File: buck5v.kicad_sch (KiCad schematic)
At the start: 11 parts, among them U4 LM76005

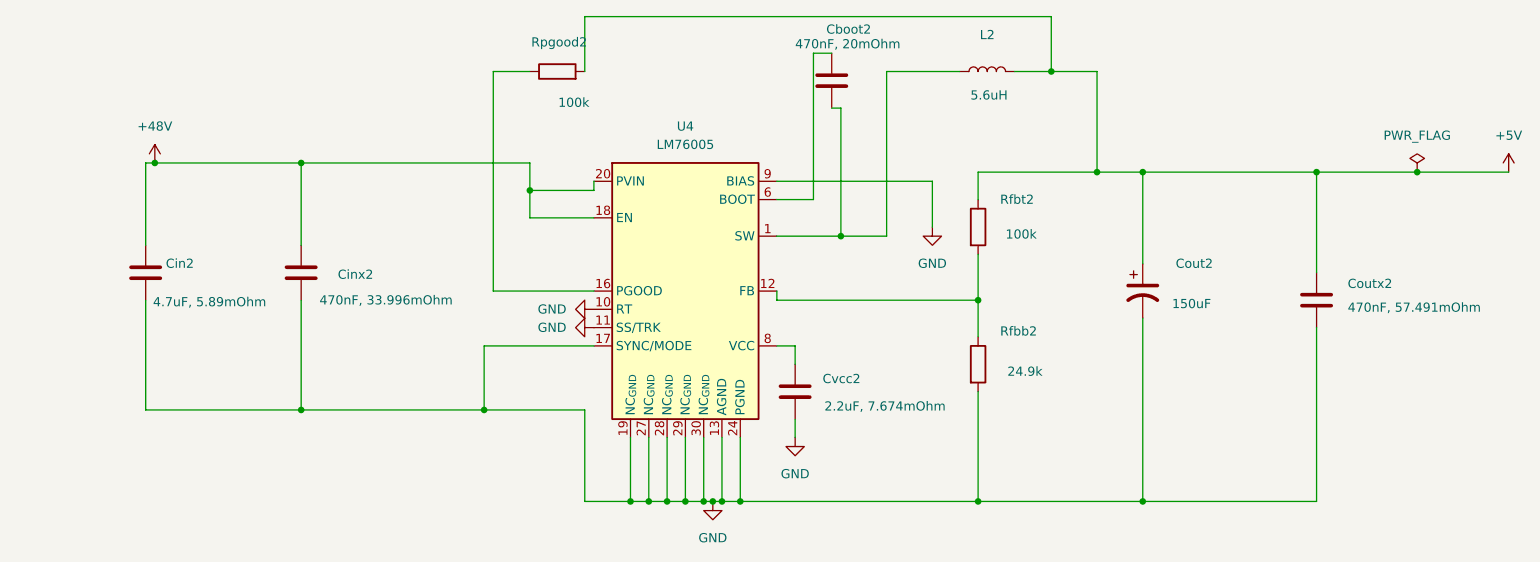
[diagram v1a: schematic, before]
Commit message: Fixed Schematics with more cost effective IC's
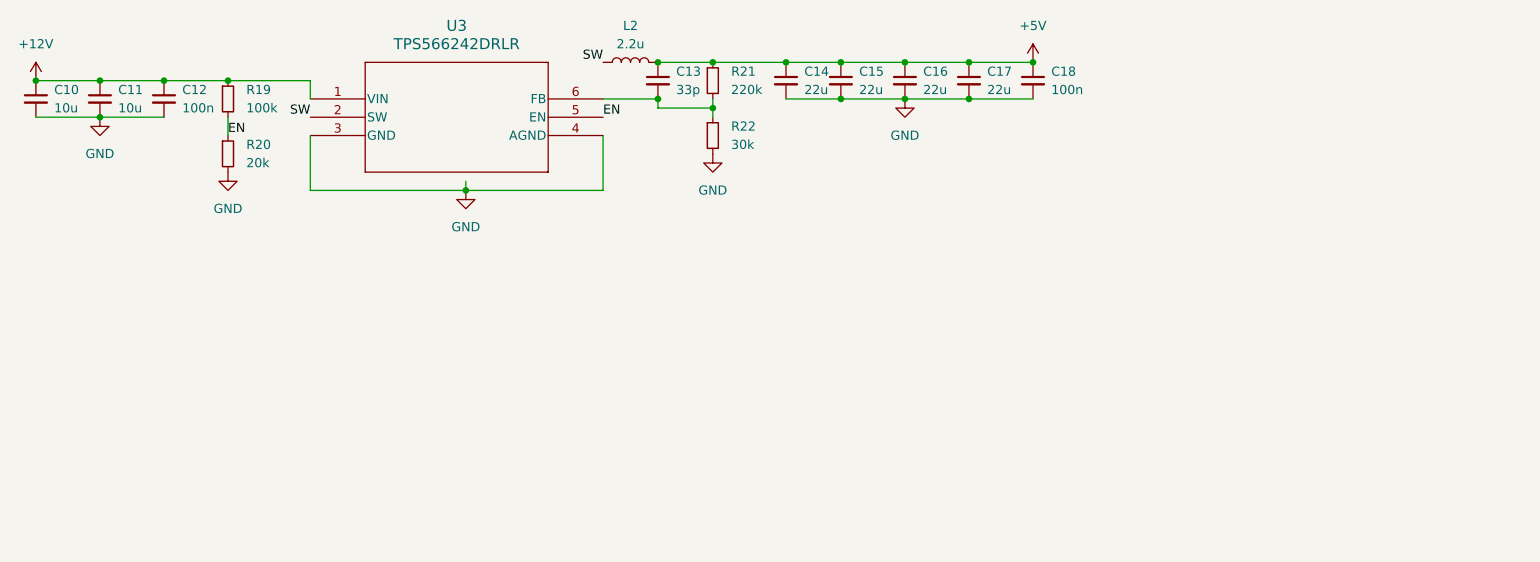
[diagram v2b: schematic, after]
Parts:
- removed Cboot2: 470nF, 20mOhm, Capacitor_SMD:C_0805_2012Metric_Pad1.18x1.45mm_HandSolder, symbol Device:C
- removed Cin2: 4.7uF, 5.89mOhm, Capacitor_SMD:C_0805_2012Metric_Pad1.18x1.45mm_HandSolder, symbol Device:C
- removed Cinx2: 470nF, 33.996mOhm, Capacitor_SMD:C_0805_2012Metric_Pad1.18x1.45mm_HandSolder, symbol Device:C
- removed Cout2: 150uF, Capacitor_SMD:C_0805_2012Metric_Pad1.18x1.45mm_HandSolder, symbol Device:C_Polarized_US
- removed Coutx2: 470nF, 57.491mOhm, Capacitor_SMD:C_0805_2012Metric_Pad1.18x1.45mm_HandSolder, symbol Device:C
- removed Cvcc2: 2.2uF, 7.674mOhm, Capacitor_SMD:C_0805_2012Metric_Pad1.18x1.45mm_HandSolder, symbol Device:C
- removed Rfbb2: 24.9k, Resistor_SMD:R_0201_0603Metric, symbol Device:R
- removed Rfbt2, Rpgood2: 100k, Resistor_SMD:R_0201_0603Metric, symbol Device:R
- removed U4: LM76005, Package_DFN_QFN:Texas_RNP0030B_WQFN-30-1EP_4x6mm_P0.5mm_EP1.8x4.5mm, symbol Regulator_Switching:LM76005
- added C10, C11: 10u, symbol Device:C_Small
- added C12, C18: 100n, symbol Device:C_Small
- added C13: 33p, symbol Device:C_Small
- added C14, C15, C16, C17: 22u, symbol Device:C_Small
- added R19: 100k, symbol Device:R_Small
- added R20: 20k, symbol Device:R_Small
- added R21: 220k, symbol Device:R_Small
- added R22: 30k, symbol Device:R_Small
- added U3: TPS566242DRLR, footprints:SOT5x3_DRL_TEX, symbol TPS566242DRLR:TPS566242DRLR
- L2: value 5.6uH -> 2.2u; footprint Inductor_SMD:L_6.3x6.3_H3 -> (none)
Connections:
- net +5V: now also C13.1, C14.1, C15.1, C16.1, C17.1, C18.1, R21.1
- net GND: now also C10.2, C11.2, C12.2, C14.2, C15.2, C16.2, C17.2, C18.2, R20.2, R22.2, U3.3 (GND), U3.4 (AGND)
- net SW: now reaches L2.1
- net SW: now also U3.2 (SW)
- new net: C13.2, R21.2, R22.1, U3.6 (FB)
- new net +12V: C10.1, C11.1, C12.1, R19.1, U3.1 (VIN)
- new net EN: R19.2, R20.1, U3.5 (EN)
